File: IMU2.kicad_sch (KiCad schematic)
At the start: 6 parts, among them U2 262-BMI088

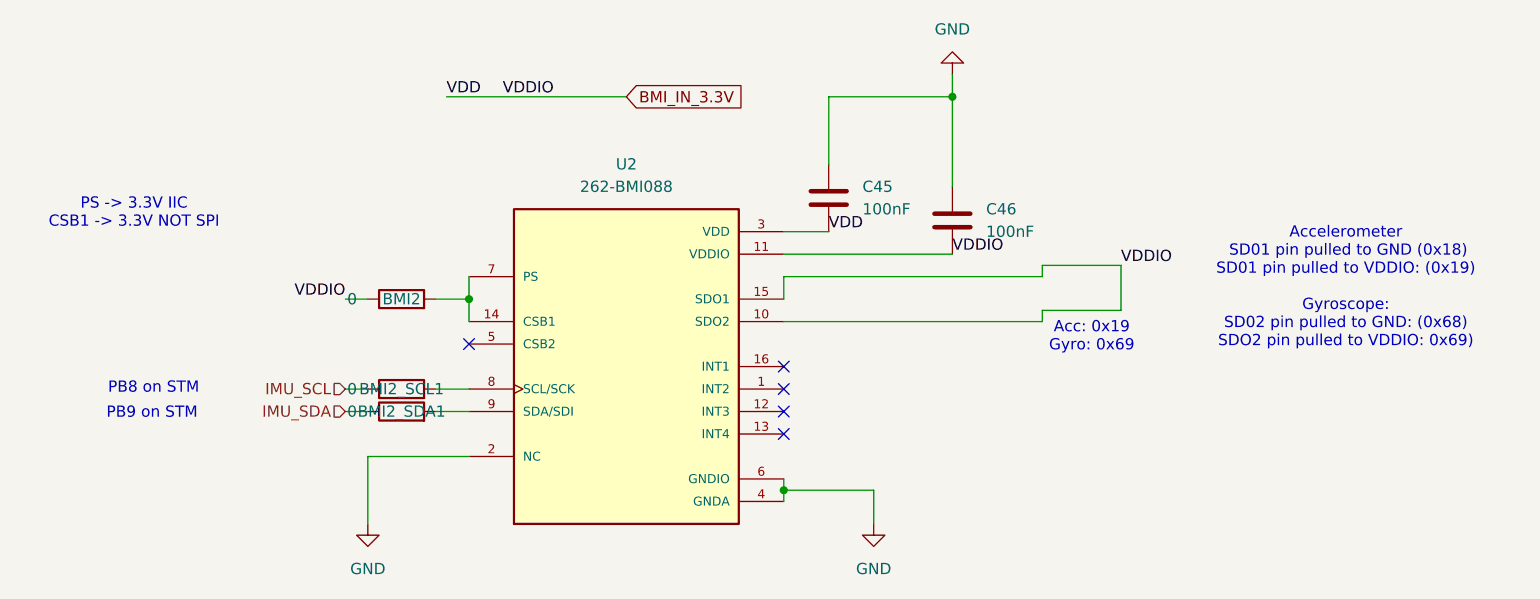
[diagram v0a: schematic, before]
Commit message: chore: Many routing changes
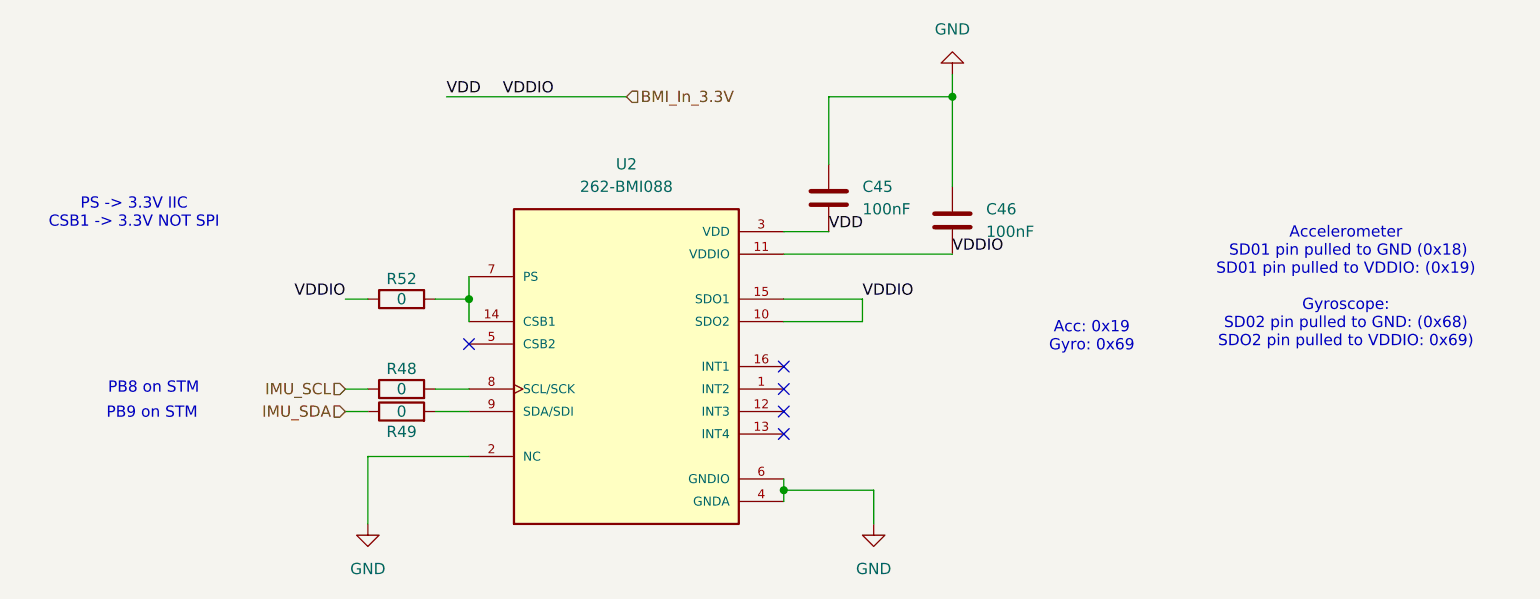
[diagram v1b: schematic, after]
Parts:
- removed BMI2, BMI2_SCL1, BMI2_SDA1: 0, Resistor_SMD:R_0603_1608Metric, symbol #dzdb:g_res/R-0-0603
- added R48, R49, R52: 0, Resistor_SMD:R_0603_1608Metric, symbol #dzdb:g_res/R-0-0603
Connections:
- net IMU_SCL: now also R48.1
- net IMU_SDA: now also R49.1
- net at U2.8 (SCL/SCK): now also R48.2
- net at U2.14 (CSB1), U2.7 (PS): now also R52.2
- net at U2.9 (SDA/SDI): now also R49.2
- net BMI_IN_3.3V renamed BMI_In_3.3V
- net BMI_In_3.3V: now also R52.1
